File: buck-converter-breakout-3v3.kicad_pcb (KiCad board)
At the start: 2 copper layers, 19.8 x 45.8 mm, 9 parts, among them J1 Conn_01x01_Pin, J2 Conn_01x02_Pin, J3 Barrel_Jack_Switch, U1 XL1509-3.3

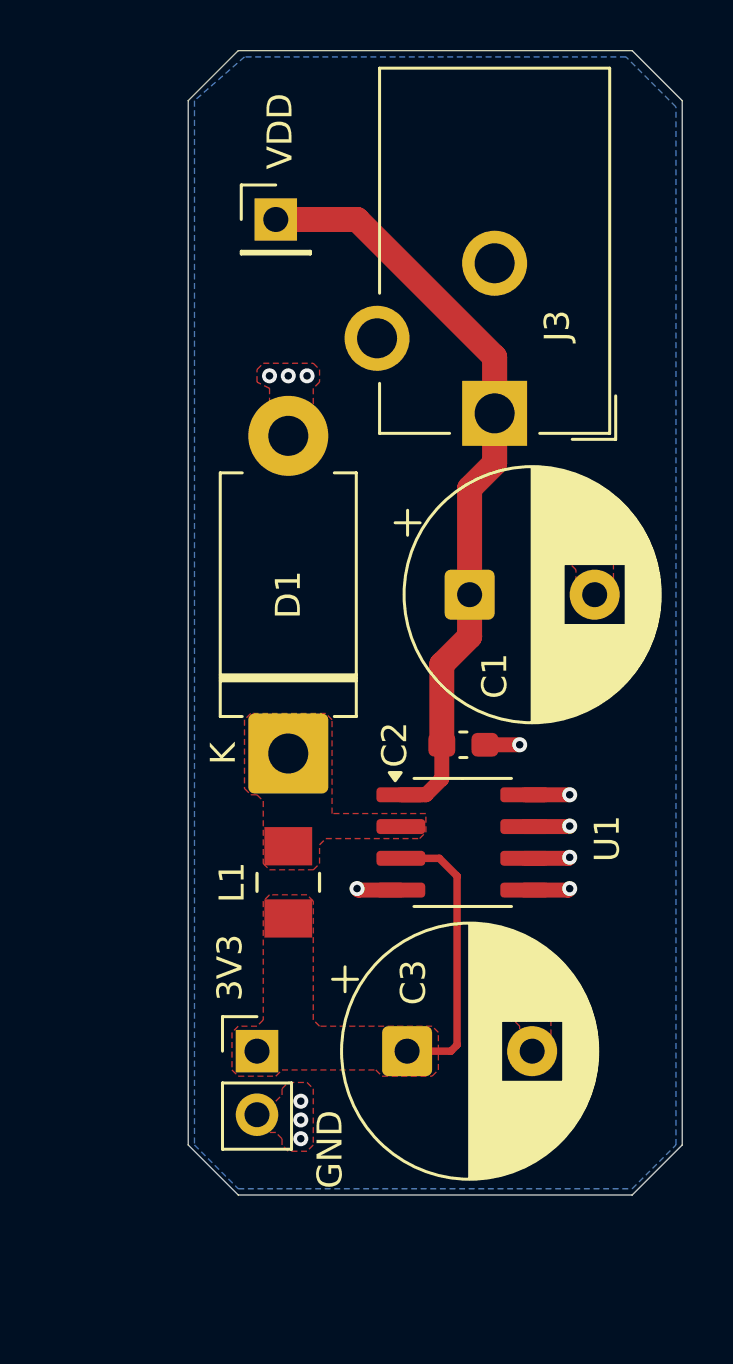
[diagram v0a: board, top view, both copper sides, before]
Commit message: ignore production files
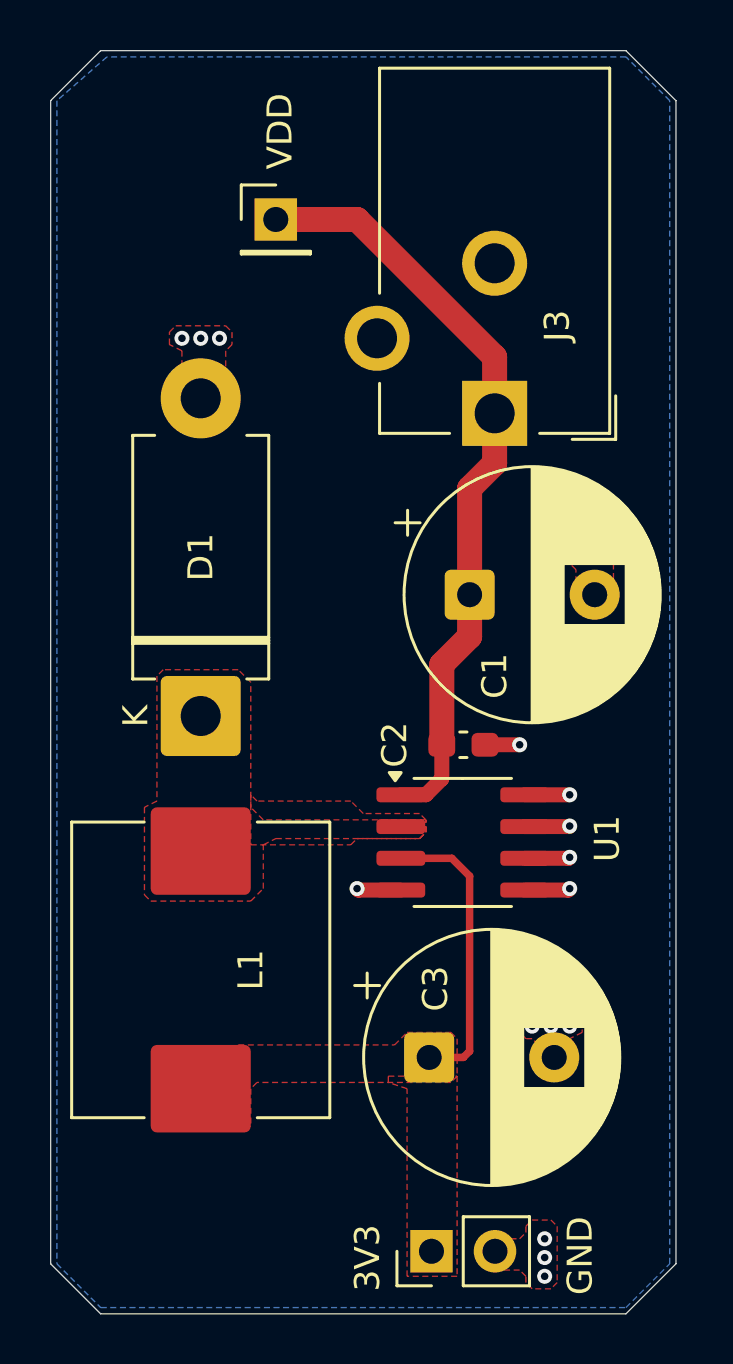
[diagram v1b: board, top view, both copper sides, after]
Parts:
- L1: footprint project_footprints:INDM3225X240N -> Inductor_SMD:L_Chilisin_BMRF00101040
- moved J2 10.6 mm to (102.5, 96.2), turned to 90 degrees
- moved L1 4.95 mm to (93.2, 85.0)
- moved D1 3.81 mm to (93.2, 74.8)
- moved C3 0.92 mm to (102.4, 88.5)
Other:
- board size 19.8 x 45.8 mm -> 25 x 50.5 mm
